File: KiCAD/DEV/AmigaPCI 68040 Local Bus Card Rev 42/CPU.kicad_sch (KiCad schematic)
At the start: 25 parts, among them J100 _BG ASSERT, U200 MC68040, U203 74LVC245

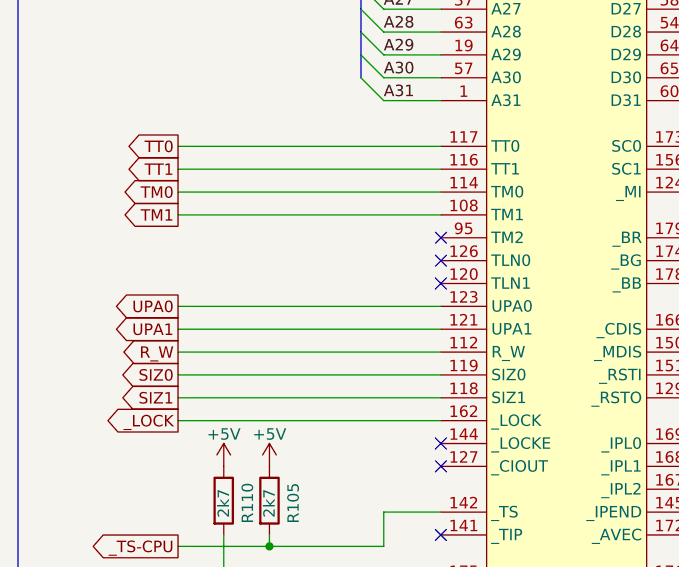
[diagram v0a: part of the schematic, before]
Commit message: Local Bus Card Rev 4.2 work.
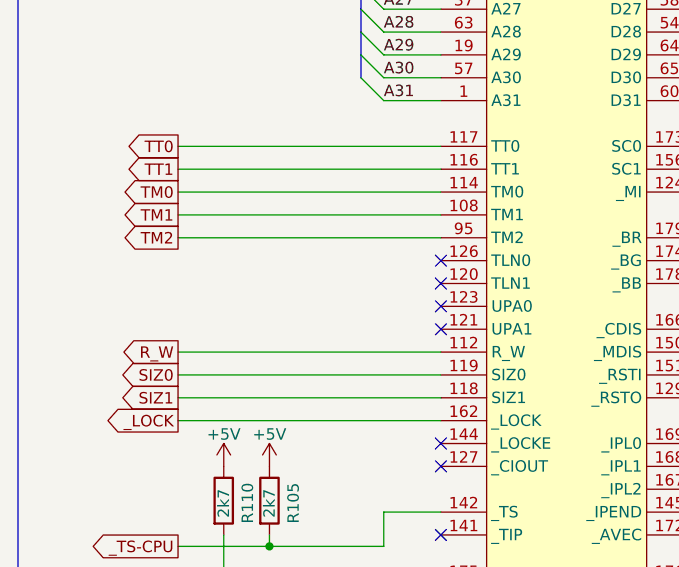
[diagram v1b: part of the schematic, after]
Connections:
- net TM2: now reaches U200.95 (TM2)
- net UPA0: no longer names the net of U200.123 (UPA0)
- net UPA1: no longer names the net of U200.121 (UPA1)
- no-connect marks 21 -> 22
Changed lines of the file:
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@@
 	(title_block
 		(title "AmigaPCI 68040 Local Bus Card")
-		(date "2025-04-03")
+		(date "2025-04-10")
 		(rev "4.2")
 	)
@@
 	)
 	(no_connect
+		(at 64.77 149.86)
+	)
+	(no_connect
 		(at 64.77 144.78)
 	)
@@
 	)
 	(no_connect
-		(at 64.77 142.24)
+		(at 64.77 152.4)
 	)
 	(no_connect
@@
 	(wire
 		(pts
-			(xy 35.56 152.4) (xy 64.77 152.4)
-		)
-		(stroke
-			(width 0)
-			(type default)
-		)
-	)
-	(wire
-		(pts
 			(xy 236.22 158.75) (xy 238.76 158.75)
 		)
@@
 	(wire
 		(pts
-			(xy 35.56 149.86) (xy 64.77 149.86)
-		)
-		(stroke
-			(width 0)
-			(type default)
-		)
-	)
-	(wire
-		(pts
 			(xy 207.01 121.92) (xy 207.01 124.46)
 		)
@@
 	(wire
 		(pts
+			(xy 35.56 142.24) (xy 64.77 142.24)
+		)
+		(stroke
+			(width 0)
+			(type default)
+		)
+	)
+	(wire
+		(pts
 			(xy 92.71 134.62) (xy 128.27 134.62)
 		)
@@
 		)
 	)
-	(global_label "TM1"
+	(global_label "TM2"
 		(shape output)
-		(at 35.56 139.7 180)
+		(at 35.56 142.24 180)
 		(fields_autoplaced yes)
 		(effects
@@
 		)
 		(property "Intersheetrefs" "${INTERSHEET_REFS}"
-			(at 29.0257 139.7 0)
+			(at 28.9463 142.24 0)
 			(effects
 				(font
@@
 		)
 	)
-	(global_label "_BB-3V"
+	(global_label "TM1"
 		(shape output)
-		(at 271.78 106.68 0)
+		(at 35.56 139.7 180)
 		(fields_autoplaced yes)
 		(effects
@@
 				(size 1.27 1.27)
 			)
-			(justify left)
+			(justify right)
 		)
 		(property "Intersheetrefs" "${INTERSHEET_REFS}"
-			(at 282.1433 106.68 0)
+			(at 29.0257 139.7 0)
 			(effects
 				(font
 					(size 1.27 1.27)
 				)
-				(justify left)
+				(justify right)
 			)
 		)
 	)
-	(global_label "R_W-3V"
+	(global_label "_BB-3V"
 		(shape output)
-		(at 271.78 101.6 0)
+		(at 271.78 106.68 0)
+		(fields_autoplaced yes)
 		(effects
 			(font
@@
 		)
 		(property "Intersheetrefs" "${INTERSHEET_REFS}"
-			(at 282.194 101.346 0)
+			(at 282.1433 106.68 0)
 			(effects
 				(font
@@
 		)
 	)
-	(global_label "UPA0"
+	(global_label "R_W-3V"
 		(shape output)
-		(at 35.56 149.86 180)
-		(fields_autoplaced yes)
+		(at 271.78 101.6 0)
 		(effects
 			(font
 				(size 1.27 1.27)
 			)
-			(justify right)
+			(justify left)
 		)
 		(property "Intersheetrefs" "${INTERSHEET_REFS}"
-			(at 27.7556 149.86 0)
+			(at 282.194 101.346 0)
 			(effects
 				(font
 					(size 1.27 1.27)
 				)
-				(justify right)
+				(justify left)
 			)
 		)
@@
 			)
 		)
-	)
-	(global_label "UPA1"
-		(shape output)
-		(at 35.56 152.4 180)
-		(fields_autoplaced yes)
-		(effects
-			(font
-				(size 1.27 1.27)
-			)
-			(justify right)
-		)
-		(property "Intersheetrefs" "${INTERSHEET_REFS}"
-			(at 27.7556 152.4 0)
-			(effects
-				(font
-					(size 1.27 1.27)
-				)
-				(justify right)
-			)
-		)
